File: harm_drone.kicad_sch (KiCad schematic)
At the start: 19 parts, among them IC1 Microcontroller, J1 SYS_DEBUG

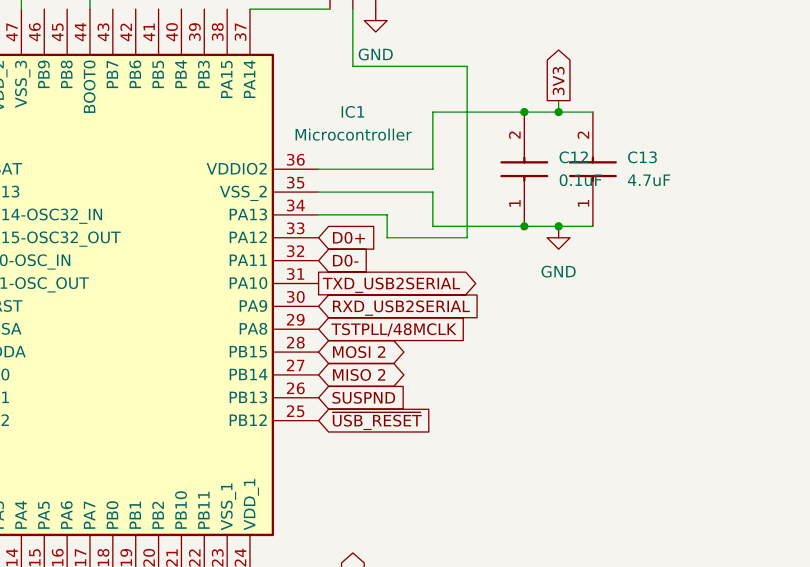
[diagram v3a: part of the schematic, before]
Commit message: USB stack changes
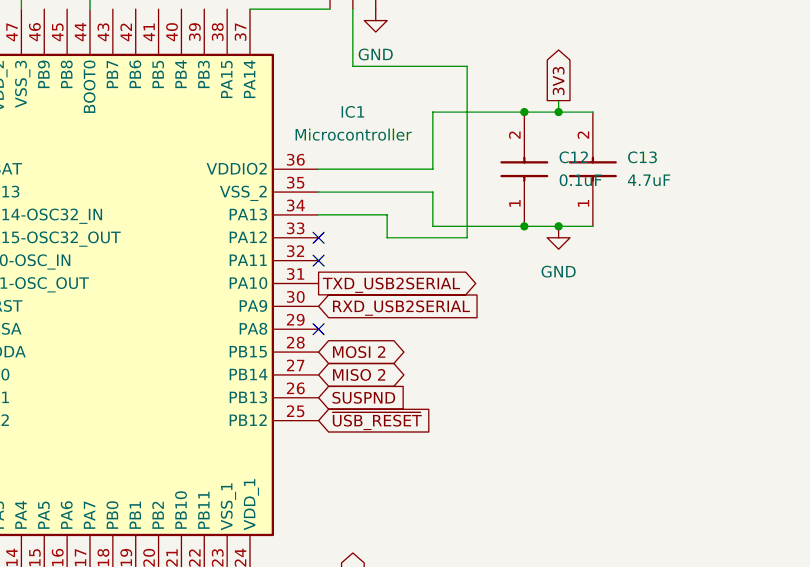
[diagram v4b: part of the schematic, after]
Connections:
- net D0+: no longer names the net of IC1.33 (PA12)
- net D0-: no longer names the net of IC1.32 (PA11)
- net TSTPLL/48MCLK: no longer names the net of IC1.29 (PA8)
- no-connect marks 0 -> 3
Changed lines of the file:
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@@
 		(color 0 0 0 0)
+	)
+	(no_connect
+		(at 161.29 115.57)
+	)
+	(no_connect
+		(at 161.29 105.41)
+	)
+	(no_connect
+		(at 161.29 107.95)
 	)
 	(wire
@@
 		)
 	)
-	(global_label "D0-"
-		(shape input)
-		(at 161.29 107.95 0)
-		(effects
-			(font
-				(size 1.27 1.27)
-			)
-			(justify left)
-		)
-		(property "Intersheetrefs" "${INTERSHEET_REFS}"
-			(at 161.29 107.95 0)
-			(effects
-				(font
-					(size 1.27 1.27)
-				)
-				(hide yes)
-			)
-		)
-	)
 	(global_label "3V3"
 		(shape output)
@@
 		)
 	)
-	(global_label "D0+"
-		(shape input)
-		(at 161.29 105.41 0)
-		(effects
-			(font
-				(size 1.27 1.27)
-			)
-			(justify left)
-		)
-		(property "Intersheetrefs" "${INTERSHEET_REFS}"
-			(at 161.29 105.41 0)
-			(effects
-				(font
-					(size 1.27 1.27)
-				)
-				(hide yes)
-			)
-		)
-	)
 	(global_label "SPI CLOCK 1"
 		(shape input)
@@
 				(hide yes)
 			)
-		)
-	)
-	(global_label "TSTPLL/48MCLK"
-		(shape input)
-		(at 161.29 115.57 0)
-		(effects
-			(font
-				(size 1.27 1.27)
-			)
-			(justify left)
-		)
-		(property "Intersheetrefs" "${INTERSHEET_REFS}"
-			(at 161.29 115.57 90)
-			(effects
-				(font
-					(size 1.27 1.27)
-				)
-				(justify left)
-				(hide yes)
-			)
